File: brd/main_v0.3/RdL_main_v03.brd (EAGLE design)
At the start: 45 x 33.7 mm, 33 parts, among them U1 MPU-6000QFN-24

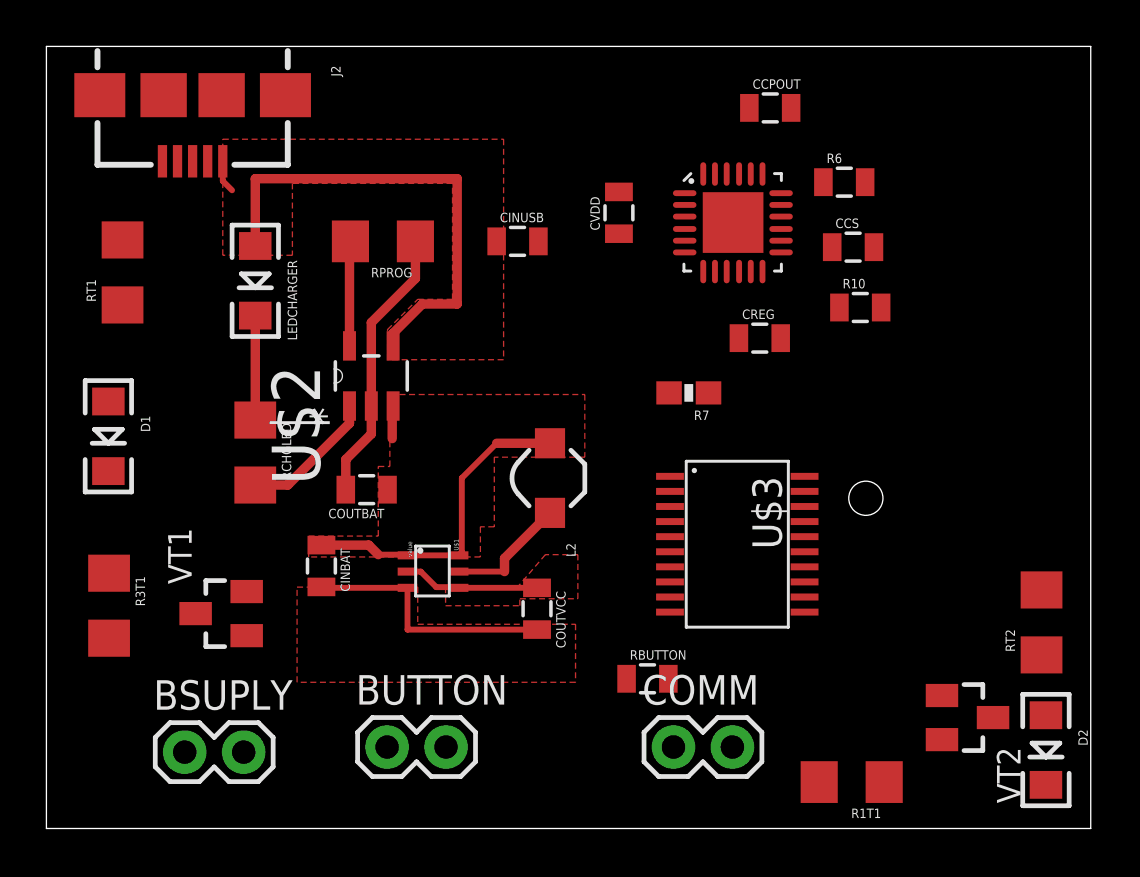
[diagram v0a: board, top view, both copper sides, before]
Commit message: Version Ready for fabrication
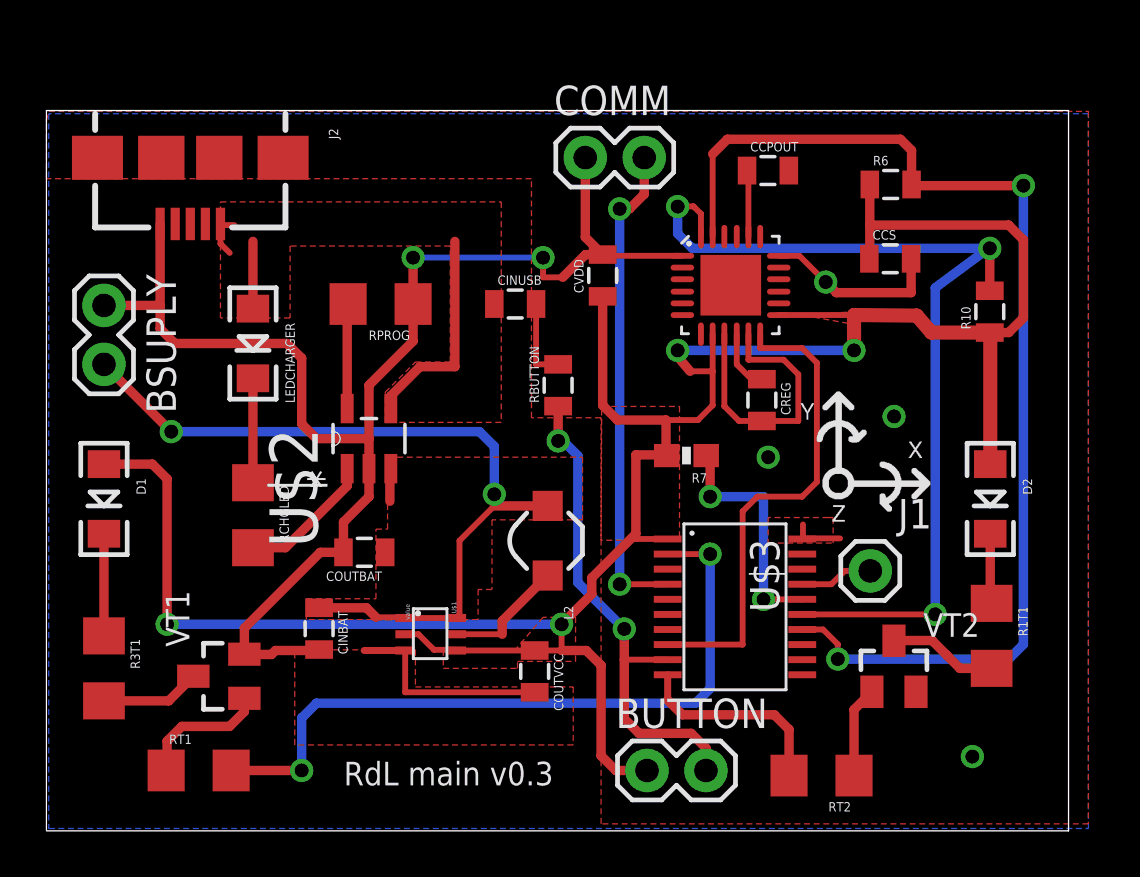
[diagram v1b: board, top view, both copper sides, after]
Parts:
- removed TEST: PRG, SparkFun-Connectors:1X01_POGOPIN_HOLE_0.58
- added J1: Test, SparkFun-Connectors:1X01
- moved COMM 25.7 mm to (23.2, 28.9)
- moved RT1 21.7 mm to (6.56, 2.50), turned to 0 degrees
- moved BSUPLY 19.6 mm to (2.48, 22.5), turned to 270 degrees
- moved RBUTTON 13.2 mm to (22.1, 19.1), turned to 90 degrees
- moved RT2 11.6 mm to (33.4, 2.28), turned to 180 degrees
- moved BUTTON 11.2 mm to (25.9, 2.50)
- moved D2 11.1 mm to (40.7, 14.2)
- moved R1T1 8.72 mm to (40.7, 8.30), turned to 270 degrees
- moved R10 5.58 mm to (40.6, 22.3), turned to 90 degrees
- moved VT2 3.86 mm to (36.5, 6.99), turned to 0 degrees
- moved CVDD 2.79 mm to (24.0, 23.8)
- moved R3T1 2.71 mm to (2.48, 6.90)
- moved D1 2.71 mm to (2.48, 14.2)
- moved J2 2.70 mm to (6.20, 28.9)
- moved LEDCHARGER 2.70 mm to (8.90, 20.9)
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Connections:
- net N$4: now also J1.1; no longer TEST.1
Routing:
- net VCC: track 5.87 -> 111.6 mm, vias 0 -> 4
- net GND: track 23.1 -> 95.6 mm, vias 0 -> 6
- net N$22: track 0.00 -> 49.4 mm, vias 0 -> 2
- net N$20: track 0.00 -> 41.6 mm, vias 0 -> 3
- net N$10: track 0.00 -> 31.1 mm, vias 0 -> 2
- net N$1: track 0.00 -> 21.7 mm, vias 0 -> 2
- net N$15: track 0.00 -> 21.1 mm, vias 0 -> 2
- net N$18: track 0.00 -> 21.1 mm
- net N$2: track 15.3 -> 35.6 mm, vias 0 -> 2
- net N$12: track 0.00 -> 10.2 mm, vias 0 -> 2
- net N$11: track 0.00 -> 8.83 mm
- net N$5: track 22.2 -> 14.1 mm
- net N$8: track 0.00 -> 5.74 mm
- net N$6: track 0.00 -> 4.72 mm
- net N$14: track 0.00 -> 4.40 mm
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- added copper zone on layer 16, net GND
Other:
- board size 45 x 33.7 mm -> 44 x 31 mm
- board text added: "RdL main v0.3"
